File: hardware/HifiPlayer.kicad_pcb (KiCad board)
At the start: 2 copper layers, 39 x 102.8 mm, 26 parts, among them J1 Conn_01x04_Female, U1 ATtiny85-20PU

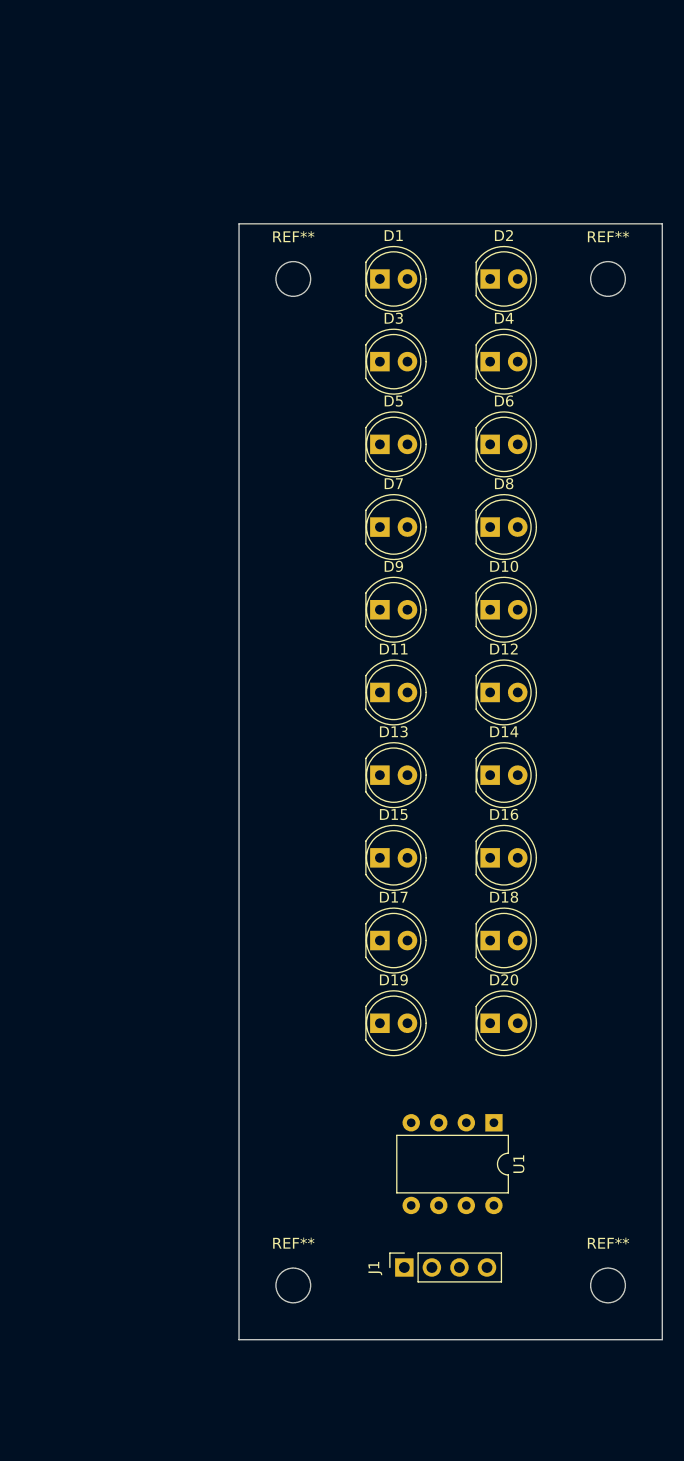
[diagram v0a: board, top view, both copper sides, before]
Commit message: First layout
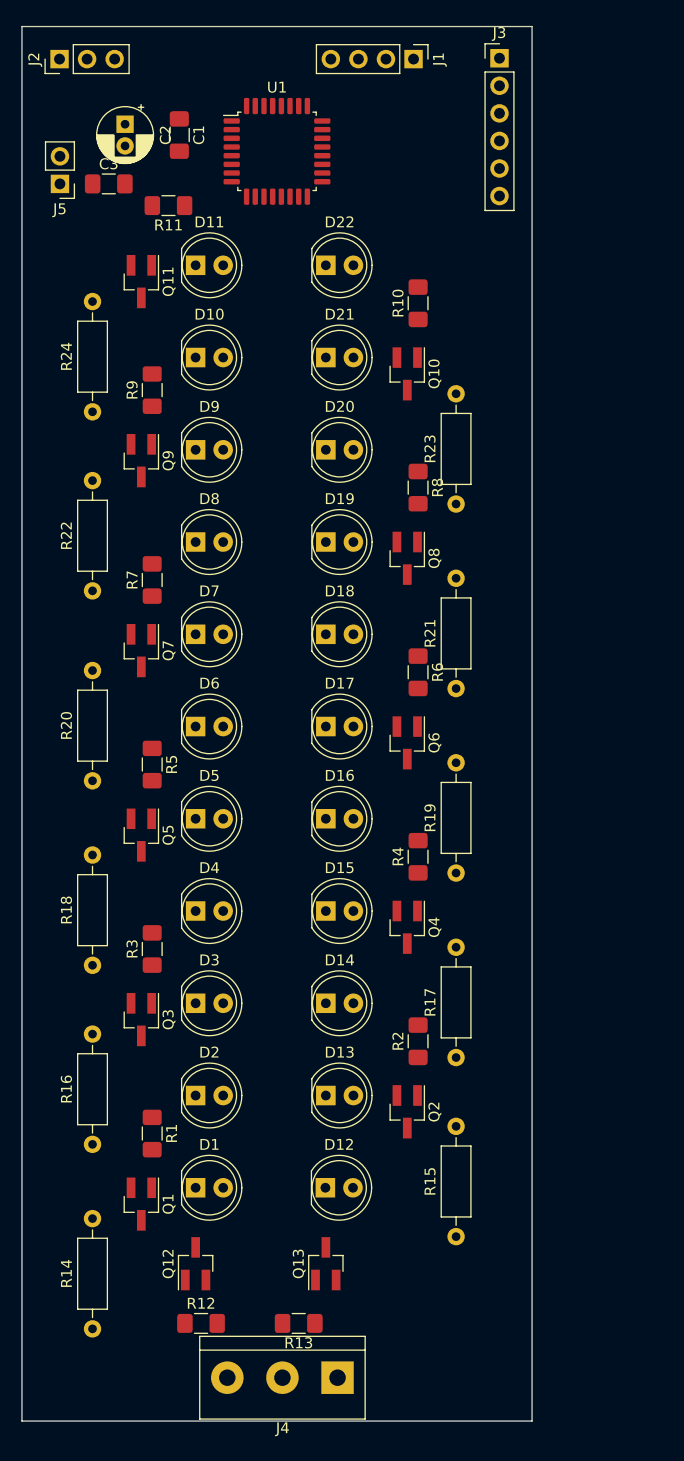
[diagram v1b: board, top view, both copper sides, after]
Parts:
- removed REF** (x4): MountingHole_3.2mm_M3_ISO7380, MountingHole:MountingHole_3.2mm_M3_ISO7380
- added C1: 100n, Capacitor_SMD:C_1206_3216Metric_Pad1.42x1.75mm_HandSolder, F.Cu at (75.5, 35.0)
- added C2: 4.7u, Capacitor_THT:CP_Radial_D5.0mm_P2.00mm, F.Cu at (70.5, 34.0)
- added C3: 100n, Capacitor_SMD:C_1206_3216Metric_Pad1.42x1.75mm_HandSolder, F.Cu at (69.0, 39.5)
- added D21: LED_RED, LED_THT:LED_D5.0mm, F.Cu at (89.0, 55.5)
- added D22: LED_RED, LED_THT:LED_D5.0mm, F.Cu at (89.0, 47.0)
- added J2: Conn_01x03_Male, Connector_PinHeader_2.54mm:PinHeader_1x03_P2.54mm_Vertical, F.Cu at (64.5, 28.0)
- added J3: Conn_01x06_Male, Connector_PinHeader_2.54mm:PinHeader_1x06_P2.54mm_Vertical, F.Cu at (105.0, 27.9)
- added J4: Screw_Terminal_01x03, TerminalBlock:TerminalBlock_bornier-3_P5.08mm, F.Cu at (90.1, 149.5)
- added J5: Conn_01x02_Male, Connector_PinHeader_2.54mm:PinHeader_1x02_P2.54mm_Vertical, F.Cu at (64.5, 39.5)
- added Q1: 2N7002K, Package_TO_SOT_SMD:SOT-23_Handsoldering, F.Cu at (72.0, 133.5)
- added Q10: 2N7002K, Package_TO_SOT_SMD:SOT-23_Handsoldering, F.Cu at (96.5, 57.0)
- added Q11: 2N7002K, Package_TO_SOT_SMD:SOT-23_Handsoldering, F.Cu at (72.0, 48.5)
- added Q12: IRLML0030, Package_TO_SOT_SMD:SOT-23_Handsoldering, F.Cu at (77.0, 139.0)
- added Q13: IRLML0030, Package_TO_SOT_SMD:SOT-23_Handsoldering, F.Cu at (89.0, 139.0)
- added Q2: 2N7002K, Package_TO_SOT_SMD:SOT-23_Handsoldering, F.Cu at (96.5, 125.0)
- added Q3: 2N7002K, Package_TO_SOT_SMD:SOT-23_Handsoldering, F.Cu at (72.0, 116.5)
- added Q4: 2N7002K, Package_TO_SOT_SMD:SOT-23_Handsoldering, F.Cu at (96.5, 108.0)
- added Q5: 2N7002K, Package_TO_SOT_SMD:SOT-23_Handsoldering, F.Cu at (72.0, 99.5)
- added Q6: 2N7002K, Package_TO_SOT_SMD:SOT-23_Handsoldering, F.Cu at (96.5, 91.0)
- added Q7: 2N7002K, Package_TO_SOT_SMD:SOT-23_Handsoldering, F.Cu at (72.0, 82.5)
- added Q8: 2N7002K, Package_TO_SOT_SMD:SOT-23_Handsoldering, F.Cu at (96.5, 74.0)
- added Q9: 2N7002K, Package_TO_SOT_SMD:SOT-23_Handsoldering, F.Cu at (72.0, 65.0)
- added R1: 100, Resistor_SMD:R_1206_3216Metric_Pad1.42x1.75mm_HandSolder, F.Cu at (73.0, 127.0)
- added R10: 100, Resistor_SMD:R_1206_3216Metric_Pad1.42x1.75mm_HandSolder, F.Cu at (97.5, 50.5)
- added R11: 100, Resistor_SMD:R_1206_3216Metric_Pad1.42x1.75mm_HandSolder, F.Cu at (74.5, 41.5)
- added R12: 100, Resistor_SMD:R_1206_3216Metric_Pad1.42x1.75mm_HandSolder, F.Cu at (77.5, 144.5)
- added R13: 100, Resistor_SMD:R_1206_3216Metric_Pad1.42x1.75mm_HandSolder, F.Cu at (86.5, 144.5)
- added R14: 220, Resistor_THT:R_Axial_DIN0207_L6.3mm_D2.5mm_P10.16mm_Horizontal, F.Cu at (67.5, 145.0)
- added R15: 220, Resistor_THT:R_Axial_DIN0207_L6.3mm_D2.5mm_P10.16mm_Horizontal, F.Cu at (101.0, 136.5)
- added R16: 220, Resistor_THT:R_Axial_DIN0207_L6.3mm_D2.5mm_P10.16mm_Horizontal, F.Cu at (67.5, 128.0)
- added R17: 220, Resistor_THT:R_Axial_DIN0207_L6.3mm_D2.5mm_P10.16mm_Horizontal, F.Cu at (101.0, 120.0)
- added R18: 220, Resistor_THT:R_Axial_DIN0207_L6.3mm_D2.5mm_P10.16mm_Horizontal, F.Cu at (67.5, 111.5)
- added R19: 220, Resistor_THT:R_Axial_DIN0207_L6.3mm_D2.5mm_P10.16mm_Horizontal, F.Cu at (101.0, 103.0)
- added R2: 100, Resistor_SMD:R_1206_3216Metric_Pad1.42x1.75mm_HandSolder, F.Cu at (97.5, 118.5)
- added R20: 220, Resistor_THT:R_Axial_DIN0207_L6.3mm_D2.5mm_P10.16mm_Horizontal, F.Cu at (67.5, 94.5)
- added R21: 220, Resistor_THT:R_Axial_DIN0207_L6.3mm_D2.5mm_P10.16mm_Horizontal, F.Cu at (101.0, 86.0)
- added R22: 220, Resistor_THT:R_Axial_DIN0207_L6.3mm_D2.5mm_P10.16mm_Horizontal, F.Cu at (67.5, 77.0)
- added R23: 220, Resistor_THT:R_Axial_DIN0207_L6.3mm_D2.5mm_P10.16mm_Horizontal, F.Cu at (101.0, 69.0)
- added R24: 220, Resistor_THT:R_Axial_DIN0207_L6.3mm_D2.5mm_P10.16mm_Horizontal, F.Cu at (67.5, 60.5)
- added R3: 100, Resistor_SMD:R_1206_3216Metric_Pad1.42x1.75mm_HandSolder, F.Cu at (73.0, 110.0)
- added R4: 100, Resistor_SMD:R_1206_3216Metric_Pad1.42x1.75mm_HandSolder, F.Cu at (97.5, 101.5)
- added R5: 100, Resistor_SMD:R_1206_3216Metric_Pad1.42x1.75mm_HandSolder, F.Cu at (73.0, 93.0)
- added R6: 100, Resistor_SMD:R_1206_3216Metric_Pad1.42x1.75mm_HandSolder, F.Cu at (97.5, 84.5)
- added R7: 100, Resistor_SMD:R_1206_3216Metric_Pad1.42x1.75mm_HandSolder, F.Cu at (73.0, 76.0)
- added R8: 100, Resistor_SMD:R_1206_3216Metric_Pad1.42x1.75mm_HandSolder, F.Cu at (97.5, 67.5)
- added R9: 100, Resistor_SMD:R_1206_3216Metric_Pad1.42x1.75mm_HandSolder, F.Cu at (73.0, 58.5)
- D1, D2, D3, D4: value LED_R -> LED_GREEN
- D10, D11, D20, D9: value LED_G -> LED_RED
- D12, D13, D14, D15, D16: value LED_G -> LED_GREEN
- D17, D18, D19: value LED_G -> LED_YELLOW
- D5: value LED_Y -> LED_GREEN
- D6, D7, D8: value LED_Y -> LED_YELLOW
- J1: value Conn_01x04_Female -> Conn_01x04_Male; footprint Connector_PinSocket_2.54mm:PinSocket_1x04_P2.54mm_Vertical -> Connector_PinHeader_2.54mm:PinHeader_1x04_P2.54mm_Vertical
- U1: value ATtiny85-20PU -> STM32G071KBTx; footprint Package_DIP:DIP-8_W7.62mm -> Package_QFP:LQFP-32_7x7mm_P0.8mm
- moved J1 111.3 mm to (97.1, 28.0), turned to 270 degrees
- moved U1 91.7 mm to (84.5, 36.5), turned to 0 degrees
- moved D1 85.4 mm to (77.0, 132.0)
- moved D2 80.0 mm to (77.0, 123.5)
- moved D3 61.5 mm to (77.0, 115.0)
- moved D4 57.4 mm to (77.0, 106.5)
- moved D20 55.0 mm to (89.0, 64.0)
- moved D12 48.1 mm to (89.0, 132.0)
- moved D19 44.6 mm to (89.0, 72.5)
- moved D11 42.9 mm to (77.0, 47.0)
- moved D5 38.5 mm to (77.0, 98.0)
- moved D6 37.6 mm to (77.0, 89.5)
- moved D10 35.7 mm to (77.0, 55.5)
- moved D18 32.0 mm to (89.0, 81.0)
- moved D13 29.9 mm to (89.0, 123.5)
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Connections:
- D1 pad 1: GND_L -> Net-(D1-Pad1)
- D1 pad 2: +3_dB -> Net-(D1-Pad2)
- D10 pad 1: GND_R -> Net-(D1-Pad1)
- D10 pad 2: -1_dB -> Net-(D10-Pad2)
- D11 pad 1: GND_L -> Net-(D1-Pad1)
- D11 pad 2: -3_dB -> Net-(D11-Pad2)
- D12 pad 1: GND_R -> Net-(D12-Pad1)
- D12 pad 2: -3_dB -> Net-(D1-Pad2)
- D13 pad 1: GND_L -> Net-(D12-Pad1)
- D13 pad 2: -5_dB -> Net-(D13-Pad2)
- D14 pad 1: GND_R -> Net-(D12-Pad1)
- D14 pad 2: -5_dB -> Net-(D14-Pad2)
- D15 pad 1: GND_L -> Net-(D12-Pad1)
- D15 pad 2: -7_dB -> Net-(D15-Pad2)
- D16 pad 1: GND_R -> Net-(D12-Pad1)
- D16 pad 2: -7_dB -> Net-(D16-Pad2)
- D17 pad 1: GND_L -> Net-(D12-Pad1)
- D17 pad 2: -10_dB -> Net-(D17-Pad2)
- D18 pad 1: GND_R -> Net-(D12-Pad1)
- D18 pad 2: -10_dB -> Net-(D18-Pad2)
- D19 pad 1: GND_L -> Net-(D12-Pad1)
- D19 pad 2: -20_dB -> Net-(D19-Pad2)
- D2 pad 1: GND_R -> Net-(D1-Pad1)
- D2 pad 2: +3_dB -> Net-(D13-Pad2)
- D20 pad 1: GND_R -> Net-(D12-Pad1)
- D20 pad 2: -20_dB -> Net-(D20-Pad2)
- D3 pad 1: GND_L -> Net-(D1-Pad1)
- D3 pad 2: +2_dB -> Net-(D14-Pad2)
- D4 pad 1: GND_R -> Net-(D1-Pad1)
- D4 pad 2: +2_dB -> Net-(D15-Pad2)
- D5 pad 1: GND_L -> Net-(D1-Pad1)
- D5 pad 2: +1_dB -> Net-(D16-Pad2)
- D6 pad 1: GND_R -> Net-(D1-Pad1)
- D6 pad 2: +1_dB -> Net-(D17-Pad2)
- D7 pad 1: GND_L -> Net-(D1-Pad1)
- D7 pad 2: 0_dB -> Net-(D18-Pad2)
- D8 pad 1: GND_R -> Net-(D1-Pad1)
- D8 pad 2: 0_dB -> Net-(D19-Pad2)
- D9 pad 1: GND_L -> Net-(D1-Pad1)
- D9 pad 2: -1_dB -> Net-(D20-Pad2)
- J1 pad 1: +5V -> GND
- J1 pad 2: Net-(J1-Pad2) -> I2S_SD
- J1 pad 3: Net-(J1-Pad3) -> I2S_WS
- J1 pad 4: GNDD -> I2S_CK
- U1 pad 4: GNDD -> +3V3
- U1 pad 5: Net-(J1-Pad2) -> GND
- U1 pad 6: Net-(J1-Pad3) -> Net-(C3-Pad1)
- U1 pad 7: Net-(U1-Pad7) -> /VU Meter LEDs/LEFT
- U1 pad 8: +5V -> /VU Meter LEDs/RIGHT
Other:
- board size 39 x 102.8 mm -> 47 x 128.5 mm
